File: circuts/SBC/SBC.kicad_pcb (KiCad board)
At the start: 2 copper layers, 108.2 x 124.9 mm, 369 parts, among them IC1 PIC16F15243-I_SS, J1 640456-3, J10 DE9_Plug, J11 buzzer, J13 Conn_01x04_Pin, J14 5v Power, J15 Barrel_Jack_MountingPin, J2 B5B-XH-A_LF__SN_, J3 Power, J4 DE9_Plug, J5 OSTTC060162, J6 XT60-M, J7 OSTTC060162, J8 DE9_Plug, Q1 MMBTA06, Q10 BC817, Q11 AO3400A, Q2 MMBTA06, Q3 MMBTA06, Q4 IRFS4227, Q5 MMBTA06, Q6 MMBTA06, Q7 MMBTA06, Q8 IRFS4227, SW1 SW_Push, SW2 SW_Push, SW3 SW_Push, SW4 SW_Push, SW5 SW_Push, SW6 rst, SW7 SW_Push, U1 UC3843, U10 ESP32-DEVKIT-V1, U12 L7805, U13 L7805, U14 L7809, U2 BTS7960B, U3 BTS7960B, U4 LM358DT, U5 AMS1117-3.3, U7 BTS7960B, U8 BTS7960B, U9 LM358DT

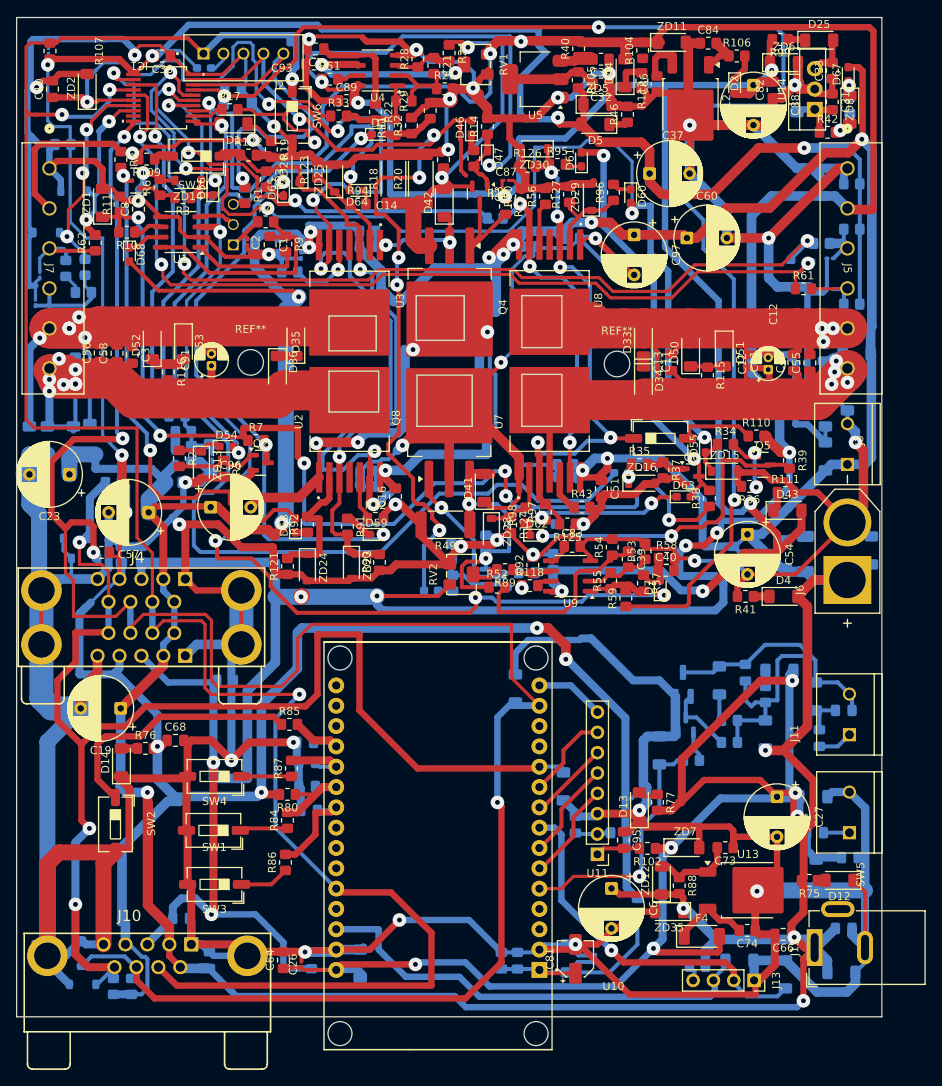
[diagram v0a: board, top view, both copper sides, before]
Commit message: siddyq done
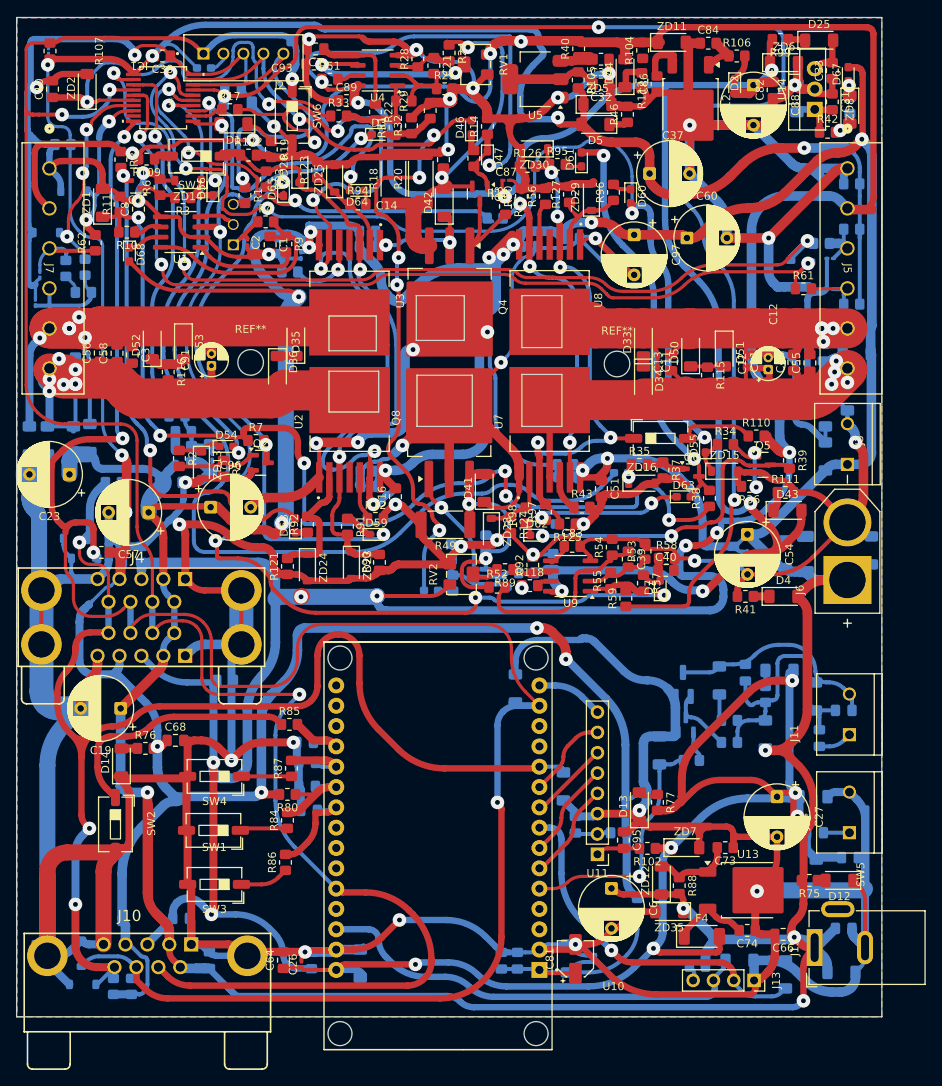
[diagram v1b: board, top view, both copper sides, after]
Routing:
- net 5v+: track 644.7 -> 634.2 mm
- net PGD: track 123.4 -> 113.5 mm
- net Mcler: track 260.3 -> 252.4 mm
- net HV: track 689.7 -> 682.2 mm
- net SCL: track 268.7 -> 262.9 mm
- net error 2: track 114.0 -> 108.4 mm
- net M1_S1: track 135.9 -> 130.4 mm
- net 9v+: track 203.6 -> 198.8 mm
- net Net-(C93-Pad1): track 28.5 -> 24.4 mm
- net M1_R: track 115.7 -> 119.6 mm
- net SDA: track 169.3 -> 165.4 mm
- net PWM: track 131.2 -> 127.3 mm
- net Motor1_OFF: track 127.4 -> 123.6 mm
- net CS: track 141.1 -> 137.6 mm
- net GND: track 1380.1 -> 1376.8 mm
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- added copper zone on B.Cu, net GND
- added copper zone on F.Cu, net GND
